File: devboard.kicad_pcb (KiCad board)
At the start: 2 copper layers, 21 x 51 mm, 34 parts, among them J1 USB_C_Receptacle_USB2.0_14P, J2 Conn_01x03, J3 Conn_01x20, J4 Conn_01x20, SW1 SW_Push, U1 RP2040, U2 NCP1117-3.3_SOT223, U3 W25Q16JVZPIQ TR, U4 MCP1700x-330xxTT, Y1 12 MHz

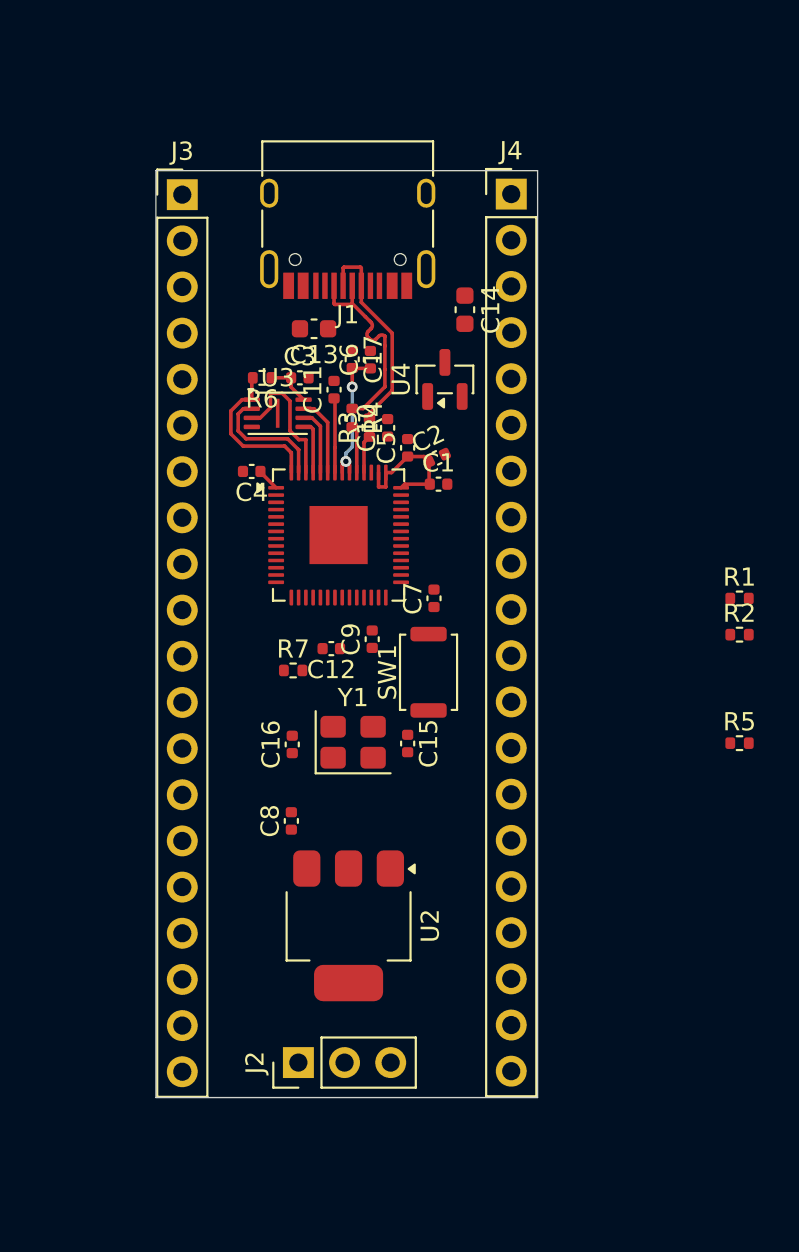
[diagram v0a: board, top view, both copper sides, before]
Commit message: routing done. i am crashing out over drc lol
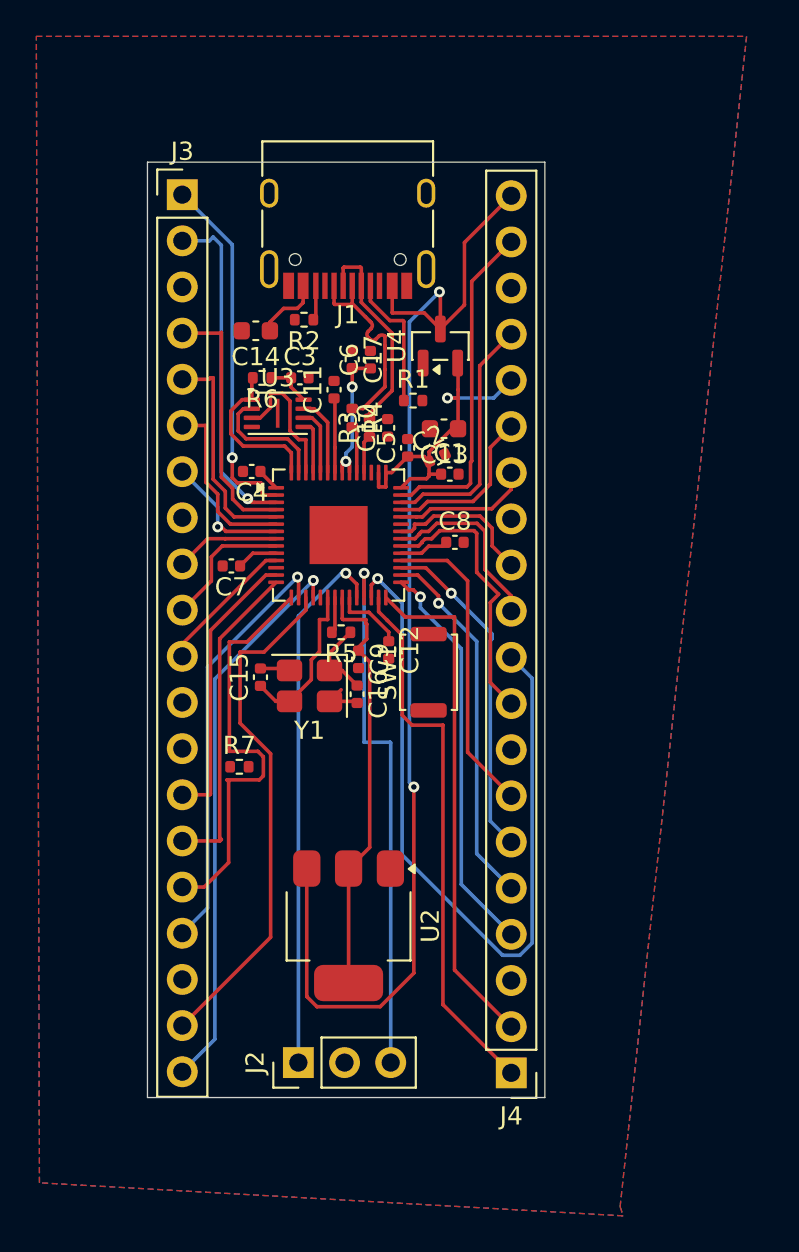
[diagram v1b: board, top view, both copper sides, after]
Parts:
- moved J4 48.4 mm to (169.7, 100.6), turned to 180 degrees
- moved R2 29.6 mm to (158.3, 59.2), turned to 180 degrees
- moved R5 22.8 mm to (160.3, 76.4), turned to 180 degrees
- moved R1 21.0 mm to (164.3, 63.6)
- moved C8 17.8 mm to (166.6, 71.5), turned to 0 degrees
- moved C14 11.6 mm to (155.6, 59.8), turned to 180 degrees
- moved C7 11.3 mm to (154.3, 72.8), turned to 180 degrees
- moved C13 9.02 mm to (166.0, 65.2)
- moved C15 8.88 mm to (155.9, 78.9), turned to 90 degrees
- moved R7 6.07 mm to (154.7, 83.8)
- moved C16 4.51 mm to (161.2, 79.8), turned to -90 degrees
- moved Y1 3.92 mm to (158.6, 79.3), turned to 180 degrees
- moved C12 3.16 mm to (163.0, 77.4), turned to -90 degrees
- moved U4 1.85 mm to (165.8, 60.6)
- moved C9 1.34 mm to (161.3, 77.9), turned to -90 degrees
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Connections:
- J4 pad 1: GPIO15 -> GPIO16
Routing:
- net VBUS: track 0.00 -> 71.4 mm, vias 0 -> 2
- net RUN: track 0.00 -> 42.9 mm, vias 0 -> 1
- net +3V3: track 19.5 -> 59.0 mm, vias 2 -> 3
- net GPIO15: track 0.00 -> 31.0 mm, vias 0 -> 1
- net GPIO16: track 0.00 -> 30.2 mm
- net SWCLK: track 0.00 -> 29.7 mm, vias 0 -> 1
- net SWD: track 0.00 -> 29.7 mm, vias 0 -> 1
- net GPIO14: track 0.00 -> 28.5 mm
- net GPIO17: track 0.00 -> 28.1 mm
- net GPIO13: track 0.00 -> 23.4 mm, vias 0 -> 1
- net GPIO12: track 0.00 -> 23.3 mm
- net GPIO18: track 0.00 -> 22.3 mm, vias 0 -> 1
- net GPIO19: track 0.00 -> 20.3 mm, vias 0 -> 1
- net GPIO0: track 0.00 -> 19.9 mm, vias 0 -> 1
- net GPIO1: track 0.00 -> 18.6 mm, vias 0 -> 1
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- added copper zone on B.Cu, net GND
- added copper zone on F.Cu, net GND
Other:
- board size 21 x 51 mm -> 21.9 x 51.5 mm
